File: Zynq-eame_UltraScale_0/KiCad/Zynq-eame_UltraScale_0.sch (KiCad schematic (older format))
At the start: 0 parts

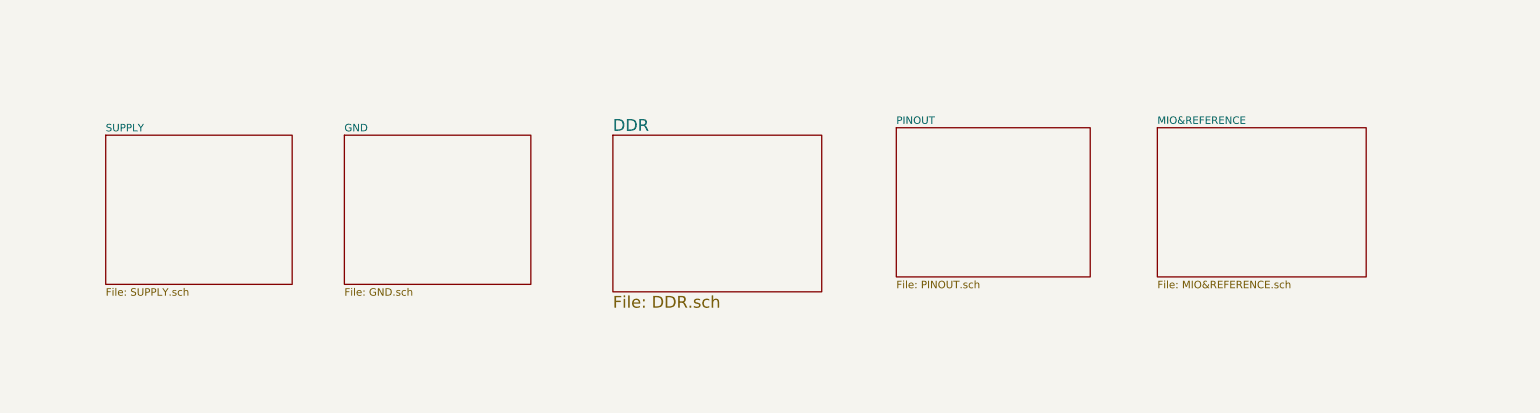
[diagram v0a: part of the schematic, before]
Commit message: UPD
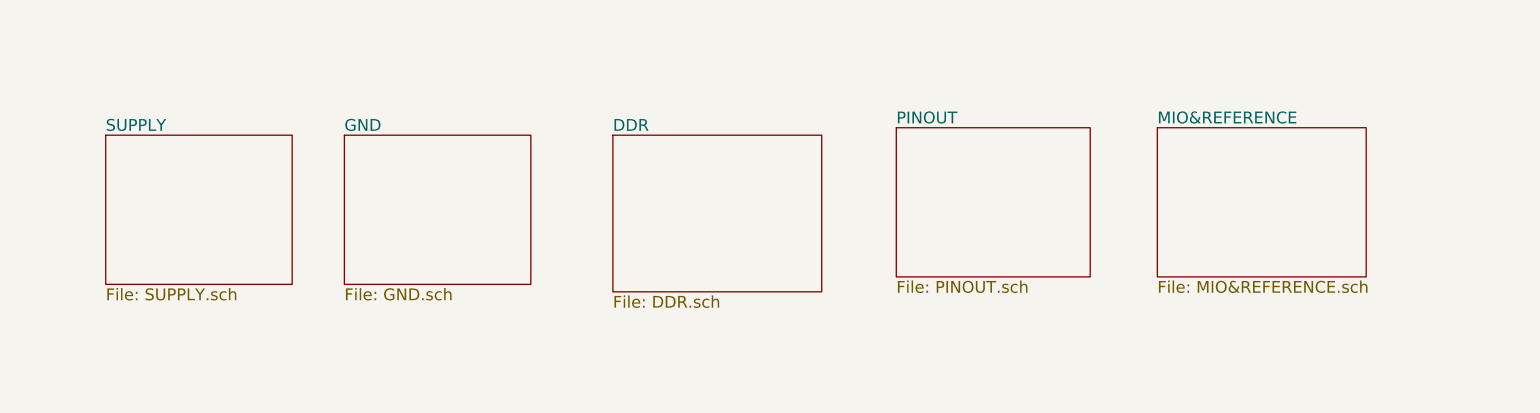
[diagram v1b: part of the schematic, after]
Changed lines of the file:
@@
 S 6250 8000 1250 1000
 U 6006A227
-F0 "SUPPLY" 50
-F1 "SUPPLY.sch" 50
+F0 "SUPPLY" 79
+F1 "SUPPLY.sch" 79
 $EndSheet
 $Sheet
 S 7850 8000 1250 1000
 U 6006A28C
-F0 "GND" 50
-F1 "GND.sch" 50
+F0 "GND" 79
+F1 "GND.sch" 79
 $EndSheet
 $Sheet
 S 11550 7950 1300 1000
 U 6006A364
-F0 "PINOUT" 50
-F1 "PINOUT.sch" 50
+F0 "PINOUT" 79
+F1 "PINOUT.sch" 79
 $EndSheet
 $Sheet
 S 13300 7950 1400 1000
 U 6006A3C1
-F0 "MIO&REFERENCE" 50
-F1 "MIO&REFERENCE.sch" 50
+F0 "MIO&REFERENCE" 79
+F1 "MIO&REFERENCE.sch" 79
 $EndSheet
 $Comp

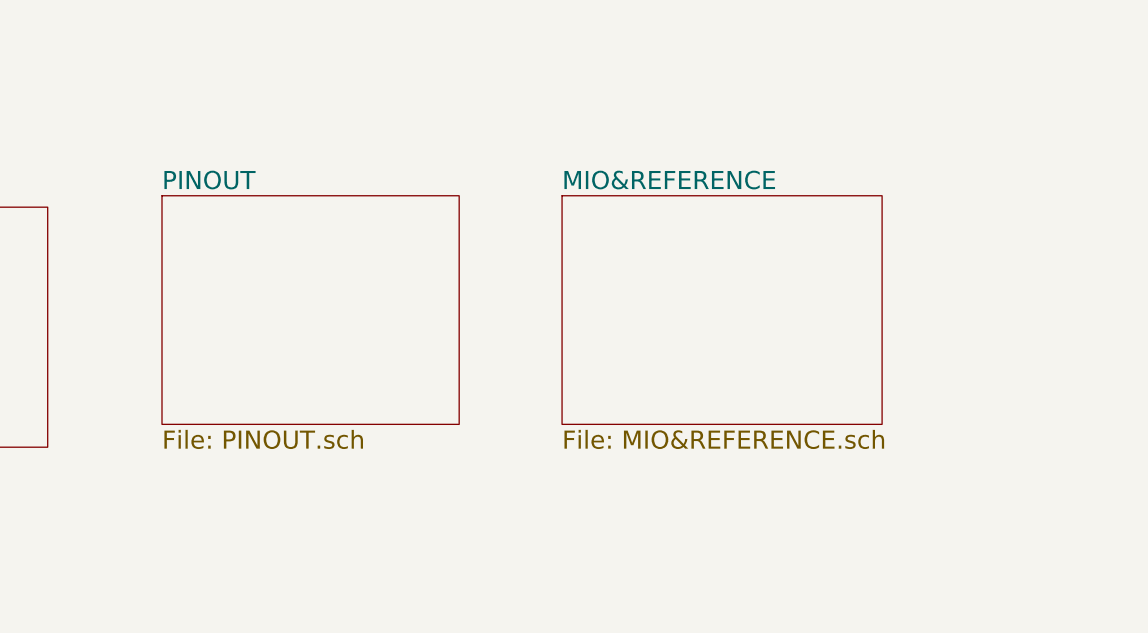
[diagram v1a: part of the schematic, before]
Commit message: upd
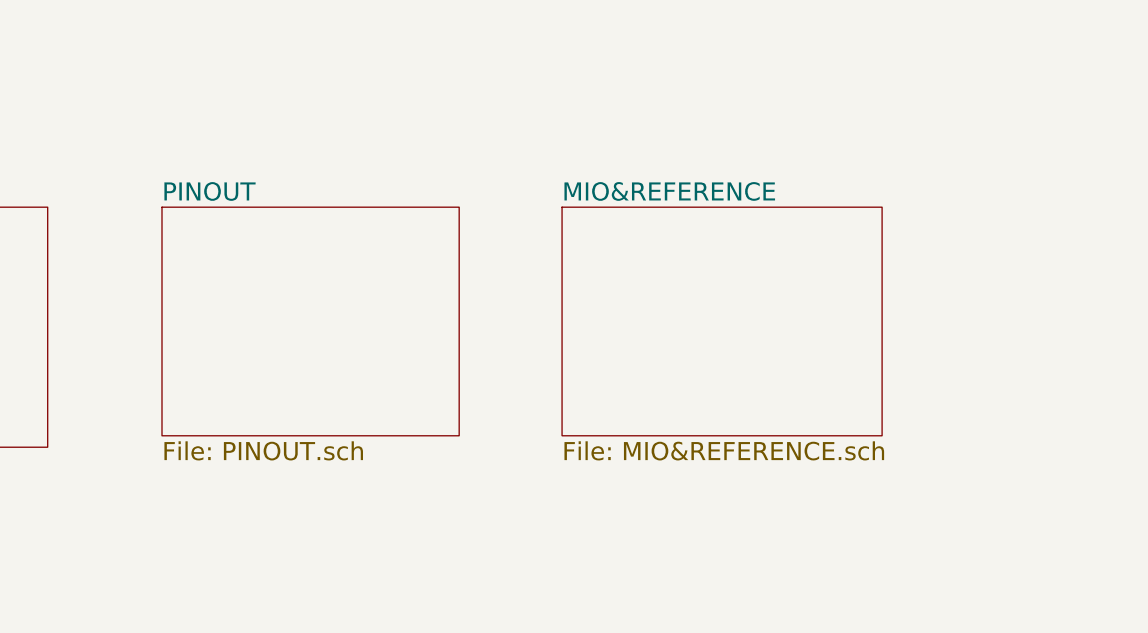
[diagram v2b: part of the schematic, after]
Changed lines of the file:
@@
 $EndSheet
 $Sheet
-S 11550 7950 1300 1000
+S 11550 8000 1300 1000
 U 6006A364
 F0 "PINOUT" 79
@@
 $EndSheet
 $Sheet
-S 13300 7950 1400 1000
+S 13300 8000 1400 1000
 U 6006A3C1
 F0 "MIO&REFERENCE" 79
